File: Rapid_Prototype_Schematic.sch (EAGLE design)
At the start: 128 parts, among them IC1 OP-AMP, IC12 LM2904ITPX/NOPB, IC2 OP-AMP, IC3 OP-AMP, IC4 LM2904ITPX/NOPB, IC5 LM2904ITPX/NOPB, IC6 LM2904ITPX/NOPB

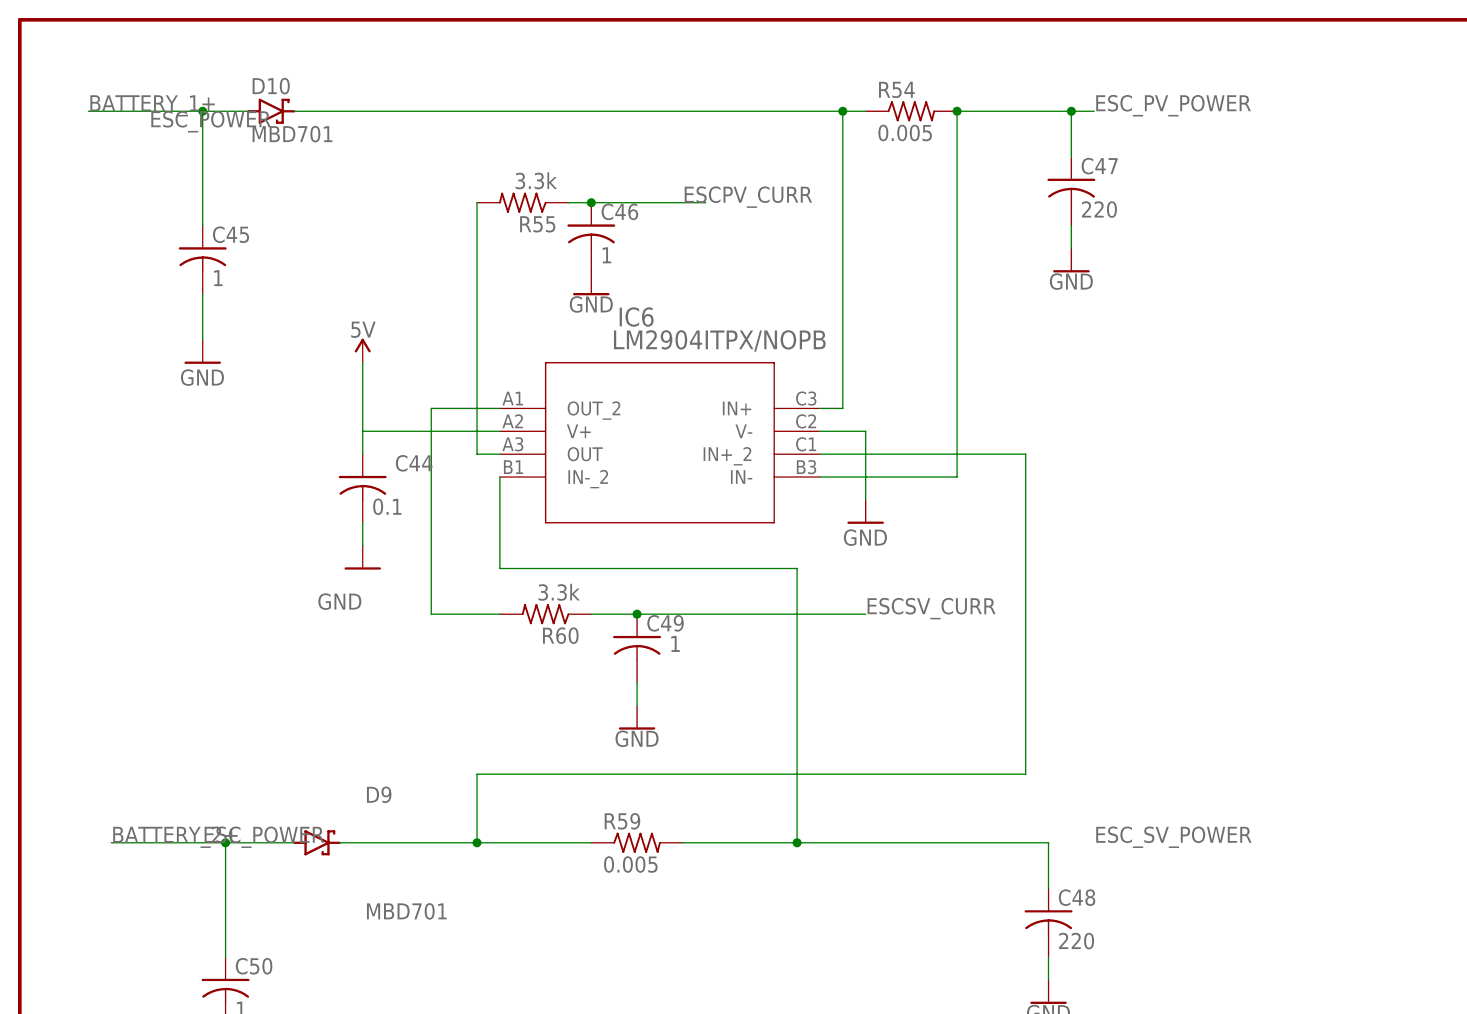
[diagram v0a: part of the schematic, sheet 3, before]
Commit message: commiting for gabe
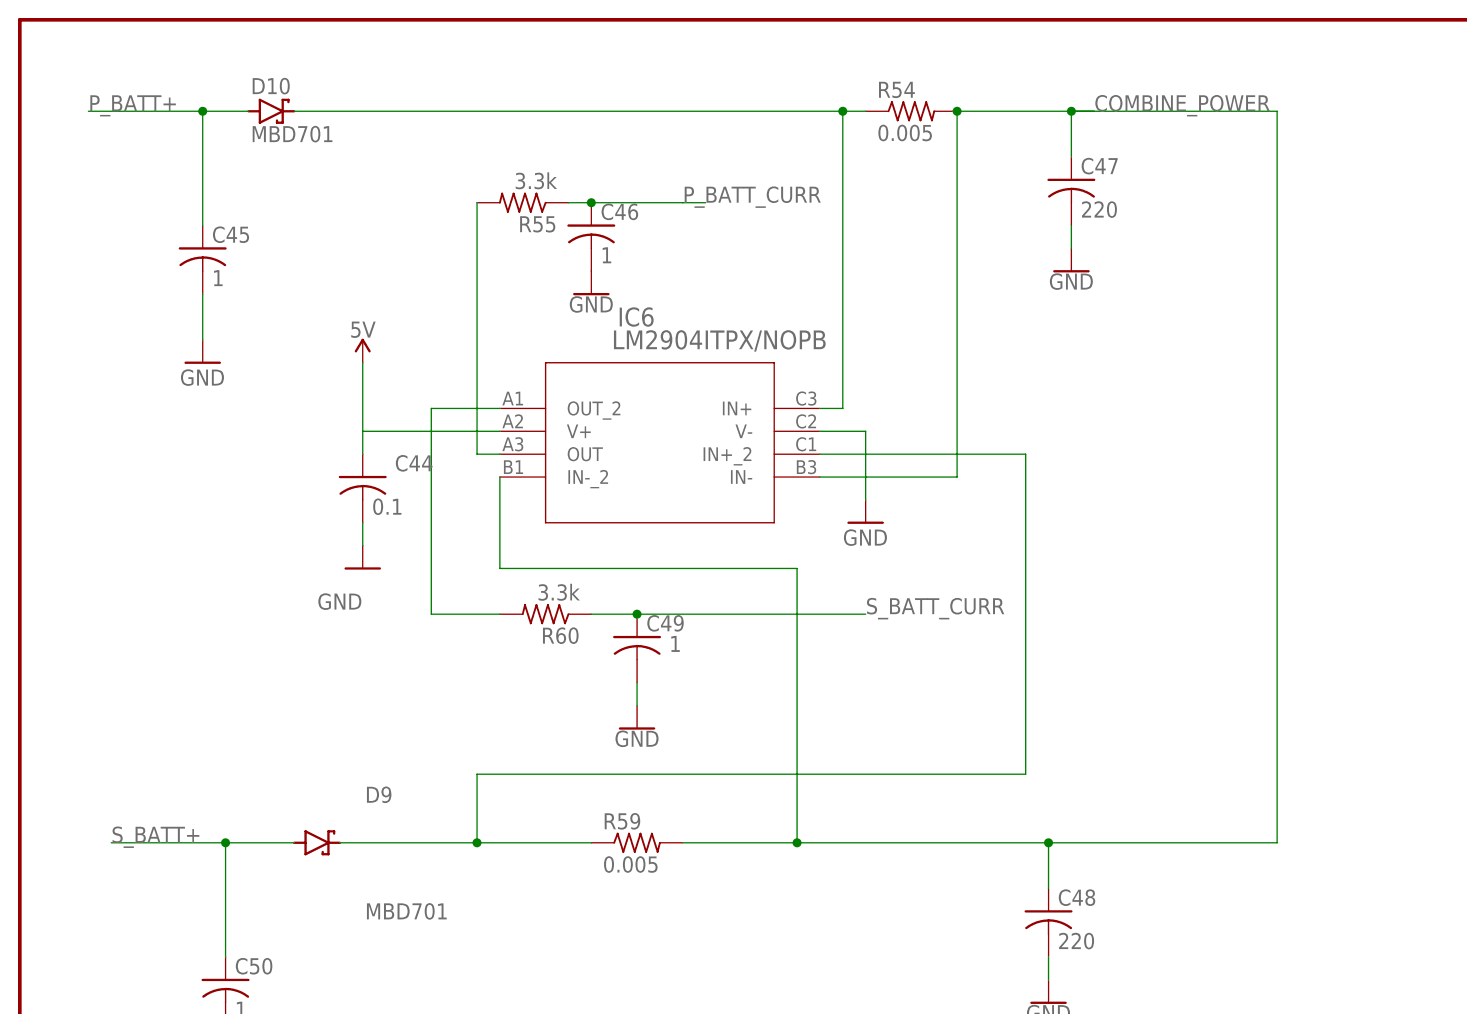
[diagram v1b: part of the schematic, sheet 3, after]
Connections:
- net BATTERY_1+ renamed P_BATT+
- net BATTERY_2+ renamed S_BATT+
- net ESCSP_SWITCH renamed ESCPF_SWITCH
- net ESCSS_SWITCH renamed ESCPA_SWITCH
- removed net ESCSFO_SWITCH: R39.1
- new net COMBINE_POWER: C47.1, C48.1, IC6.IN-, IC6.IN-_2, R54.2, R59.2
- new net ESCPV_SWITCH: R51.1
- new net P_BATT_CURR: C46.1, R55.1
- new net S_BATT_CURR: C49.1, R60.1
- net ESCPV_CURR: no longer C46.1, R55.1
- net ESCSF_SWITCH: now also R39.1; no longer R51.1
- net ESCSV_CURR: no longer C49.1, R60.1
- net ESC_PV_POWER: no longer C47.1, IC6.IN-, R54.2
- net ESC_SV_POWER: no longer C48.1, IC6.IN-_2, R59.2
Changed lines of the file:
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@@
 </segment>
 </net>
-<net name="ESCSS_SWITCH" class="0">
+<net name="ESCPA_SWITCH" class="0">
 <segment>
 <pinref part="R31" gate="G$1" pin="1"/>
@@
 </segment>
 </net>
-<net name="ESCSFO_SWITCH" class="0">
+<net name="ESCSF_SWITCH" class="0">
 <segment>
 <pinref part="R39" gate="G$1" pin="1"/>
@@
 </segment>
 </net>
-<net name="ESCSS_POWER" class="0">
+<net name="ESCPA_POWER" class="0">
 <segment>
 <wire x1="-114.3" y1="-35.56" x2="-99.06" y2="-35.56" width="0.1524" layer="91"/>
@@
 <wire x1="-25.4" y1="-35.56" x2="-10.16" y2="-35.56" width="0.1524" layer="91"/>
 <label x="-20.32" y="-35.56" size="1.778" layer="95"/>
-</segment>
-</net>
-<net name="ESCSFO_POWER" class="0">
-<segment>
-<wire x1="66.04" y1="-35.56" x2="81.28" y2="-35.56" width="0.1524" layer="91"/>
-<label x="71.12" y="-35.56" size="1.778" layer="95"/>
 </segment>
 </net>
@@
 </segment>
 </net>
-<net name="ESCSP_SWITCH" class="0">
+<net name="ESCPF_SWITCH" class="0">
 <segment>
 <pinref part="R47" gate="G$1" pin="1"/>
@@
 </segment>
 </net>
-<net name="ESCSF_SWITCH" class="0">
+<net name="ESCPV_SWITCH" class="0">
 <segment>
 <pinref part="R51" gate="G$1" pin="1"/>
@@
 <label x="25.4" y="78.74" size="1.778" layer="95"/>
 </segment>
+<segment>
+<wire x1="66.04" y1="-35.56" x2="81.28" y2="-35.56" width="0.1524" layer="91"/>
+<label x="71.12" y="-35.56" size="1.778" layer="95"/>
+</segment>
 </net>
 <net name="ESCSP_POWER" class="0">
@@
 <wire x1="-99.06" y1="83.82" x2="-160.02" y2="83.82" width="0.1524" layer="91"/>
 <junction x="-99.06" y="83.82"/>
-<label x="-162.56" y="83.82" size="1.778" layer="95" rot="R180"/>
 <pinref part="R54" gate="G$1" pin="1"/>
 <pinref part="D10" gate="1" pin="C"/>
@@
 <pinref part="R59" gate="G$1" pin="1"/>
 <wire x1="-127" y1="2.54" x2="-139.7" y2="2.54" width="0.1524" layer="91"/>
-<label x="-170.18" y="2.54" size="1.778" layer="95"/>
 <pinref part="IC6" gate="A" pin="IN+_2"/>
 <wire x1="-139.7" y1="2.54" x2="-154.94" y2="2.54" width="0.1524" layer="91"/>
@@
 </segment>
 </net>
-<net name="ESCPV_CURR" class="0">
-<segment>
-<pinref part="R55" gate="G$1" pin="1"/>
-<pinref part="C46" gate="G$1" pin="1"/>
-<wire x1="-129.54" y1="73.66" x2="-127" y2="73.66" width="0.1524" layer="91"/>
-<label x="-116.84" y="73.66" size="1.778" layer="95"/>
-<wire x1="-127" y1="73.66" x2="-114.3" y2="73.66" width="0.1524" layer="91"/>
-<junction x="-127" y="73.66"/>
-</segment>
-</net>
-<net name="ESC_PV_POWER" class="0">
-<segment>
+<net name="N$35" class="0">
+<segment>
+<pinref part="IC6" gate="A" pin="OUT_2"/>
+<wire x1="-137.16" y1="50.8" x2="-144.78" y2="50.8" width="0.1524" layer="91"/>
+<wire x1="-144.78" y1="50.8" x2="-144.78" y2="27.94" width="0.1524" layer="91"/>
+<pinref part="R60" gate="G$1" pin="2"/>
+<wire x1="-144.78" y1="27.94" x2="-137.16" y2="27.94" width="0.1524" layer="91"/>
+</segment>
+</net>
+<net name="S_BATT+" class="0">
+<segment>
+<pinref part="C50" gate="G$1" pin="1"/>
+<wire x1="-167.64" y1="-10.16" x2="-167.64" y2="2.54" width="0.1524" layer="91"/>
+<pinref part="D9" gate="1" pin="A"/>
+<wire x1="-167.64" y1="2.54" x2="-160.02" y2="2.54" width="0.1524" layer="91"/>
+<wire x1="-167.64" y1="2.54" x2="-180.34" y2="2.54" width="0.1524" layer="91"/>
+<junction x="-167.64" y="2.54"/>
+<label x="-180.34" y="2.54" size="1.778" layer="95"/>
+</segment>
+</net>
+<net name="P_BATT+" class="0">
+<segment>
+<pinref part="C45" gate="G$1" pin="1"/>
+<wire x1="-170.18" y1="71.12" x2="-170.18" y2="83.82" width="0.1524" layer="91"/>
+<pinref part="D10" gate="1" pin="A"/>
+<wire x1="-170.18" y1="83.82" x2="-165.1" y2="83.82" width="0.1524" layer="91"/>
+<wire x1="-170.18" y1="83.82" x2="-182.88" y2="83.82" width="0.1524" layer="91"/>
+<junction x="-170.18" y="83.82"/>
+<label x="-182.88" y="83.82" size="1.778" layer="95"/>
+</segment>
+</net>
+<net name="S_BATT_CURR" class="0">
+<segment>
+<pinref part="R60" gate="G$1" pin="1"/>
+<pinref part="C49" gate="G$1" pin="1"/>
+<wire x1="-127" y1="27.94" x2="-121.92" y2="27.94" width="0.1524" layer="91"/>
+<wire x1="-121.92" y1="27.94" x2="-96.52" y2="27.94" width="0.1524" layer="91"/>
+<junction x="-121.92" y="27.94"/>
+<label x="-96.52" y="27.94" size="1.778" layer="95"/>
+</segment>
+</net>
+<net name="COMBINE_POWER" class="0">
+<segment>
+<wire x1="-50.8" y1="2.54" x2="-50.8" y2="83.82" width="0.1524" layer="91"/>
 <pinref part="IC6" gate="A" pin="IN-"/>
 <wire x1="-86.36" y1="43.18" x2="-101.6" y2="43.18" width="0.1524" layer="91"/>
@@
 <wire x1="-86.36" y1="43.18" x2="-86.36" y2="83.82" width="0.1524" layer="91"/>
 <junction x="-86.36" y="83.82"/>
-</segment>
-</net>
-<net name="ESC_SV_POWER" class="0">
-<segment>
+<wire x1="-50.8" y1="83.82" x2="-73.66" y2="83.82" width="0.1524" layer="91"/>
+<pinref part="C48" gate="G$1" pin="1"/>
+<wire x1="-76.2" y1="2.54" x2="-76.2" y2="-2.54" width="0.1524" layer="91"/>
 <pinref part="R59" gate="G$1" pin="2"/>
 <wire x1="-116.84" y1="2.54" x2="-104.14" y2="2.54" width="0.1524" layer="91"/>
-<label x="-71.12" y="2.54" size="1.778" layer="95"/>
+<wire x1="-104.14" y1="2.54" x2="-76.2" y2="2.54" width="0.1524" layer="91"/>
+<junction x="-104.14" y="2.54"/>
 <pinref part="IC6" gate="A" pin="IN-_2"/>
-<wire x1="-104.14" y1="2.54" x2="-76.2" y2="2.54" width="0.1524" layer="91"/>
 <wire x1="-137.16" y1="43.18" x2="-137.16" y2="33.02" width="0.1524" layer="91"/>
 <wire x1="-137.16" y1="33.02" x2="-104.14" y2="33.02" width="0.1524" layer="91"/>
 <wire x1="-104.14" y1="33.02" x2="-104.14" y2="2.54" width="0.1524" layer="91"/>
-<junction x="-104.14" y="2.54"/>
-<pinref part="C48" gate="G$1" pin="1"/>
-<wire x1="-76.2" y1="2.54" x2="-76.2" y2="-2.54" width="0.1524" layer="91"/>
-</segment>
-</net>
-<net name="N$35" class="0">
-<segment>
-<pinref part="IC6" gate="A" pin="OUT_2"/>
-<wire x1="-137.16" y1="50.8" x2="-144.78" y2="50.8" width="0.1524" layer="91"/>
-<wire x1="-144.78" y1="50.8" x2="-144.78" y2="27.94" width="0.1524" layer="91"/>
-<pinref part="R60" gate="G$1" pin="2"/>
-<wire x1="-144.78" y1="27.94" x2="-137.16" y2="27.94" width="0.1524" layer="91"/>
-</segment>
-</net>
-<net name="ESCSV_CURR" class="0">
-<segment>
-<pinref part="R60" gate="G$1" pin="1"/>
-<pinref part="C49" gate="G$1" pin="1"/>
-<wire x1="-127" y1="27.94" x2="-121.92" y2="27.94" width="0.1524" layer="91"/>
-<wire x1="-121.92" y1="27.94" x2="-96.52" y2="27.94" width="0.1524" layer="91"/>
-<junction x="-121.92" y="27.94"/>
-<label x="-96.52" y="27.94" size="1.778" layer="95"/>
-</segment>
-</net>
-<net name="BATTERY_2+" class="0">
-<segment>
-<pinref part="C50" gate="G$1" pin="1"/>
-<wire x1="-167.64" y1="-10.16" x2="-167.64" y2="2.54" width="0.1524" layer="91"/>
-<pinref part="D9" gate="1" pin="A"/>
-<wire x1="-167.64" y1="2.54" x2="-160.02" y2="2.54" width="0.1524" layer="91"/>
-<wire x1="-167.64" y1="2.54" x2="-180.34" y2="2.54" width="0.1524" layer="91"/>
-<junction x="-167.64" y="2.54"/>
-<label x="-180.34" y="2.54" size="1.778" layer="95"/>
-</segment>
-</net>
-<net name="BATTERY_1+" class="0">
-<segment>
-<pinref part="C45" gate="G$1" pin="1"/>
-<wire x1="-170.18" y1="71.12" x2="-170.18" y2="83.82" width="0.1524" layer="91"/>
-<pinref part="D10" gate="1" pin="A"/>
-<wire x1="-170.18" y1="83.82" x2="-165.1" y2="83.82" width="0.1524" layer="91"/>
-<wire x1="-170.18" y1="83.82" x2="-182.88" y2="83.82" width="0.1524" layer="91"/>
-<junction x="-170.18" y="83.82"/>
-<label x="-182.88" y="83.82" size="1.778" layer="95"/>
-</segment>
-</net>
+<wire x1="-76.2" y1="2.54" x2="-50.8" y2="2.54" width="0.1524" layer="91"/>
+<junction x="-76.2" y="2.54"/>
+</segment>
+</net>
+<net name="P_BATT_CURR" class="0">
+<segment>
+<pinref part="R55" gate="G$1" pin="1"/>
+<pinref part="C46" gate="G$1" pin="1"/>
+<wire x1="-129.54" y1="73.66" x2="-127" y2="73.66" width="0.1524" layer="91"/>
+<label x="-116.84" y="73.66" size="1.778" layer="95"/>
+<wire x1="-127" y1="73.66" x2="-116.84" y2="73.66" width="0.1524" layer="91"/>
+<junction x="-127" y="73.66"/>
+<wire x1="-114.3" y1="73.66" x2="-116.84" y2="73.66" width="0.1524" layer="91"/>
+</segment>
+</net>
